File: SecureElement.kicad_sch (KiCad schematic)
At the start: 3 parts, among them IC8 STSAFA110S8OCD03

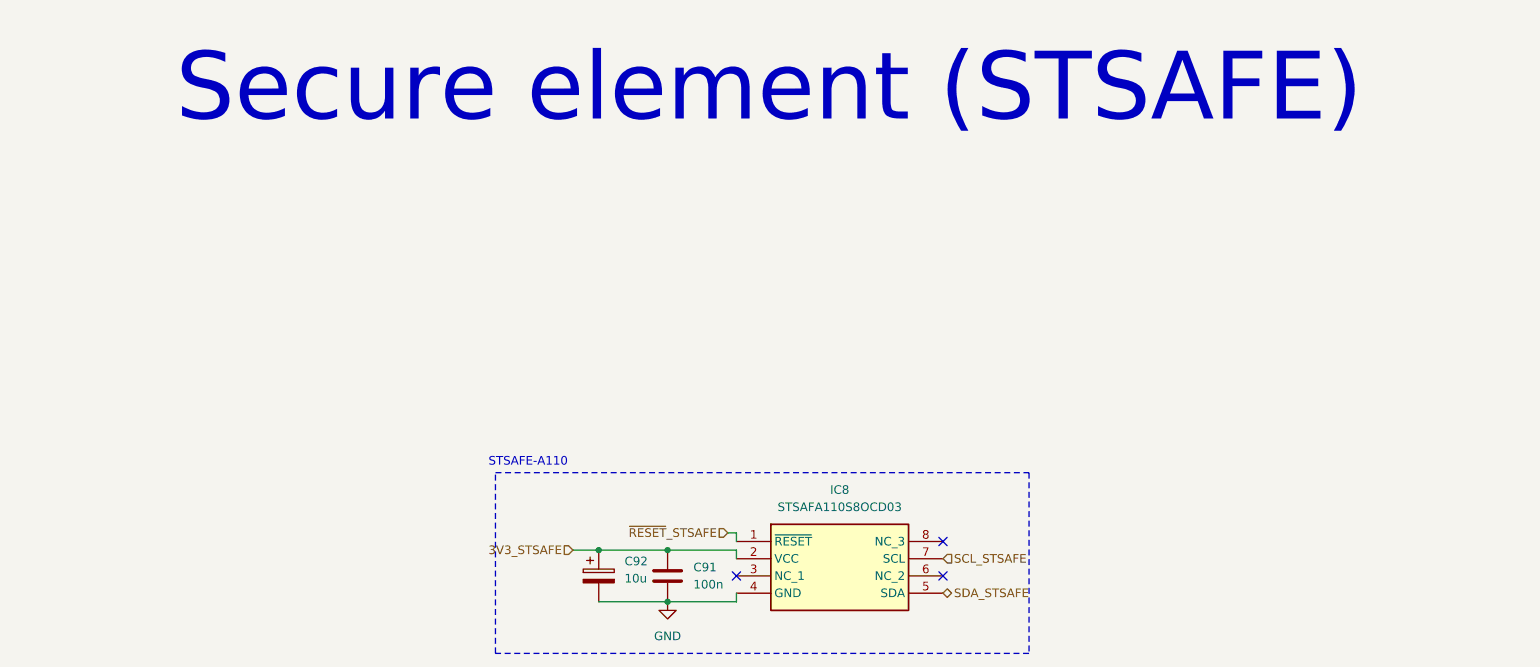
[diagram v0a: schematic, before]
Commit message: Continue schematic review
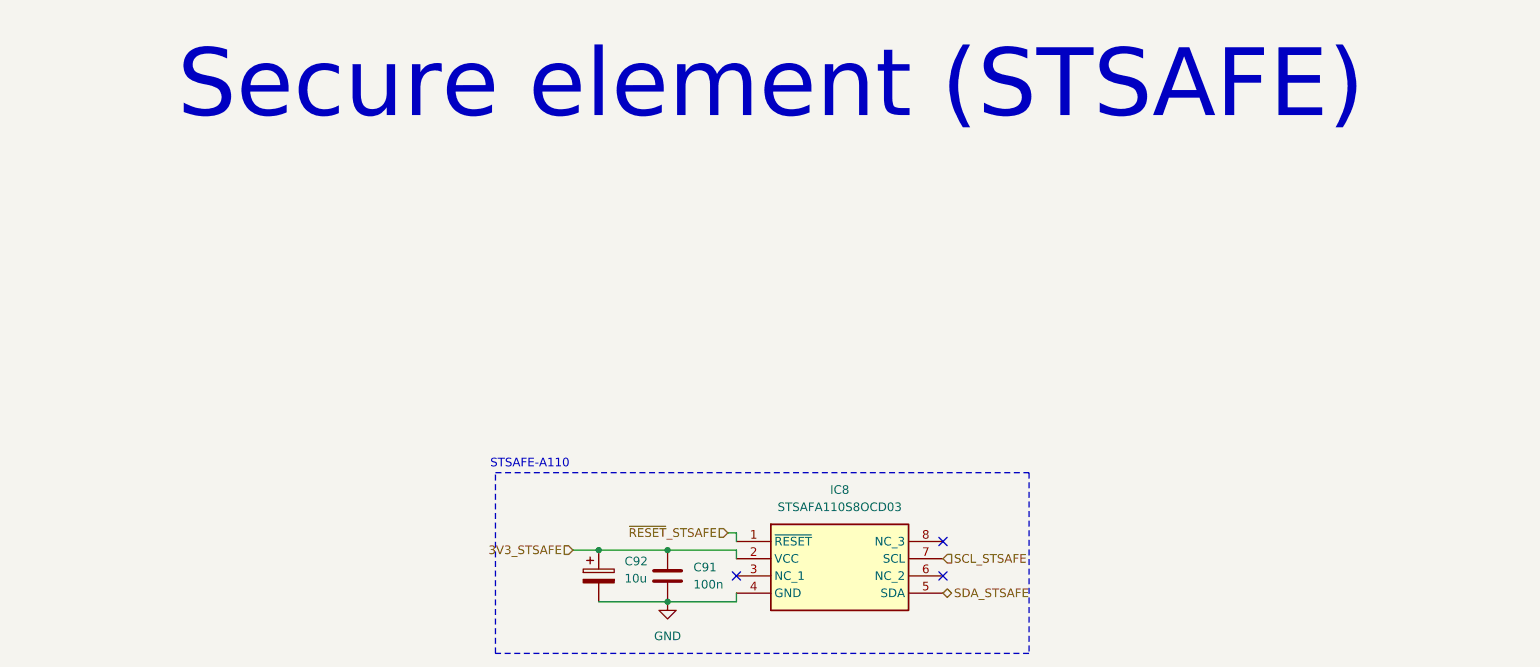
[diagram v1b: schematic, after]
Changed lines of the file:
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@@
 	(text "STSAFE-A110"
 		(exclude_from_sim no)
-		(at 105.156 78.486 0)
+		(at 105.41 78.74 0)
 		(effects
 			(font
@@
 	(text "Secure element (STSAFE)"
 		(exclude_from_sim no)
-		(at 140.716 23.368 0)
+		(at 140.97 22.86 0)
 		(effects
 			(font
